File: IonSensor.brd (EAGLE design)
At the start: 50.8 x 22.9 mm, 43 parts, among them IC1 QUAD_OPAMPD, IC2 QUAD_OPAMPD, IC3 QUAD_OPAMPD

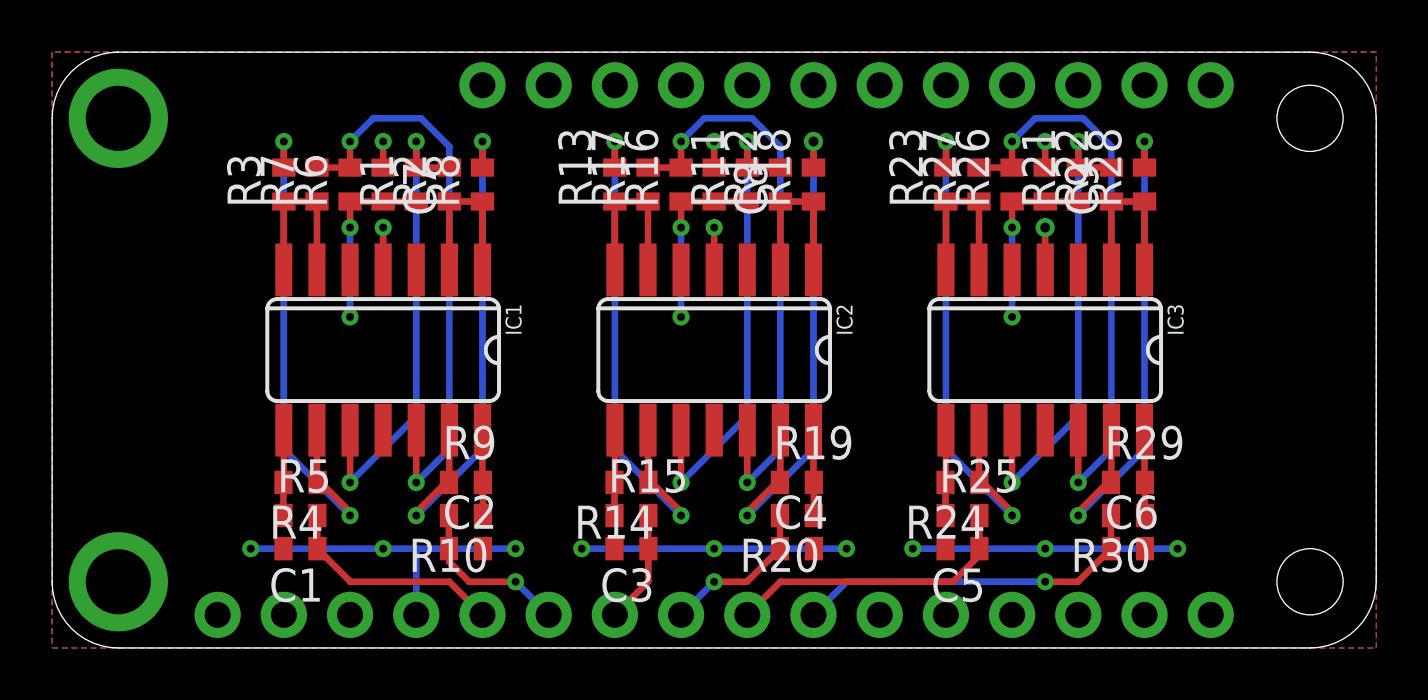
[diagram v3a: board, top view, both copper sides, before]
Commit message: Revert "Rev. D"
This reverts commit b0cd00c38bcd6b0f7db002c888a5e278bdb202ce.
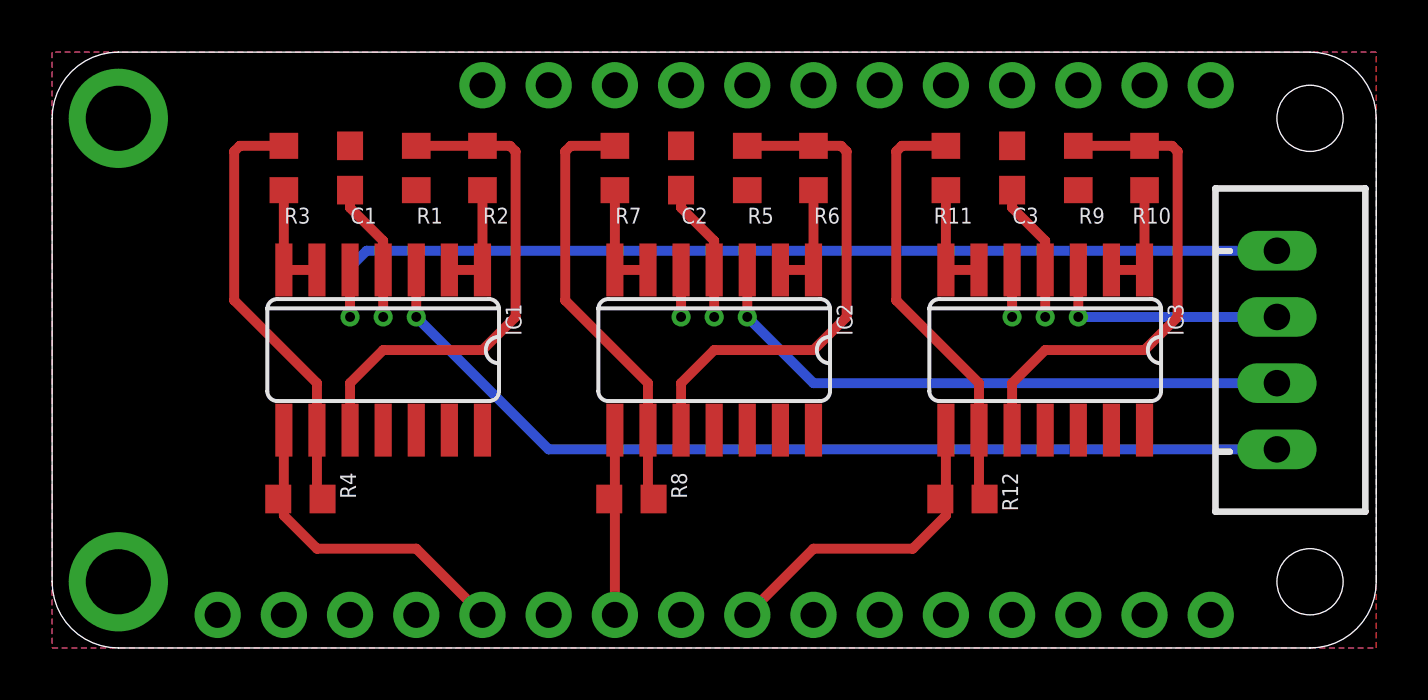
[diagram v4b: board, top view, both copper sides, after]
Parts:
- removed C4, C5, C6, C7, C8, C9: 0.1uF, adafruit:C0402
- removed R13, R17, R18, R22, R23, R27, R28: 10k, adafruit:R0402
- removed R14, R16, R19, R21, R24, R26, R29: 100k, adafruit:R0402
- removed R15, R20, R25, R30: 1M, adafruit:R0402
- added X1: JST-XH-04-PIN-LONG-PAD, Rembrandt Electronics - JST XH Connectors v1-0:JST-XH-04-PACKAGE-LONG-PAD
- C1, C2, C3: device adafruit:C0402 -> adafruit:C0603
- R1, R2, R3, R4, R7, R9: device adafruit:R0402 -> adafruit:R0603
- R10: value 1M -> 10k; device adafruit:R0402 -> adafruit:R0603
- R11, R6: value 100k -> 10k; device adafruit:R0402 -> adafruit:R0603
- R12, R8: value 10k -> 100k; device adafruit:R0402 -> adafruit:R0603
- R5: value 1M -> 100k; device adafruit:R0402 -> adafruit:R0603
- moved R10 29.3 mm to (41.9, 18.4), turned to 90 degrees
- moved R9 26.4 mm to (39.4, 18.4), turned to 90 degrees
- moved R5 21.7 mm to (26.7, 18.4), turned to 90 degrees
- moved C3 20.7 mm to (36.8, 18.4), turned to 90 degrees
- moved R6 17.8 mm to (29.2, 18.4)
- moved C2 16.8 mm to (24.1, 18.4), turned to 90 degrees
- moved C1 14.7 mm to (11.4, 18.4), turned to 90 degrees
- moved R12 13.9 mm to (34.9, 5.71), turned to 180 degrees
- moved R8 13.4 mm to (22.2, 5.71), turned to 180 degrees
- moved R7 11.4 mm to (21.6, 18.4)
- moved R11 7.65 mm to (34.3, 18.4)
- moved R2 1.42 mm to (16.5, 18.4)
- moved R4 0.63 mm to (9.53, 5.71)
- moved R1 0.63 mm to (14.0, 18.4)
- moved R3 0.63 mm to (8.89, 18.4)
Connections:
- removed net A1: C2.1, MS1.6, R10.2
- removed net A3: C4.1, MS1.8, R20.2
- removed net A5: C6.1, MS1.10, R30.2
- removed net C1+: IC1.1, IC1.2, R2.1, R8.1
- removed net C1-: IC1.6, IC1.7, R3.1, R7.1
- removed net C2+: IC2.1, IC2.2, R12.1, R18.1
- removed net C2-: IC2.6, IC2.7, R13.1, R17.1
- removed net C3+: IC3.1, IC3.2, R22.1, R28.1
- removed net C3-: IC3.6, IC3.7, R23.1, R27.1
- removed net N$10: IC1.14, R10.1, R9.2
- removed net N$15: IC3.13, R28.2, R29.1
- removed net N$16: IC2.14, R19.2, R20.1
- removed net N$17: IC3.8, R24.2, R25.1
- removed net N$18: IC3.14, R29.2, R30.1
- removed net N$4 (its old number): IC1.12, R6.2, R7.2
- removed net N$5: IC1.8, R4.2, R5.1
- new net N$1: IC1.1, IC1.2, R2.1
- net +3V3: now also C1.1, C2.1, C3.1; no longer C7.1, C8.1, C9.1
- net A0: now also IC1.8, R4.2; no longer C1.1, R5.2
- net A2: now also IC2.8, R8.2; no longer C3.1, R15.2
- net A4: now also IC3.8, R12.2; no longer C5.1, R25.2
- net CH0: now also X1.4
- net CH1: now also X1.3
- net CH2: now also X1.2
- net GND: now also R5.1, R9.1; no longer C4.2, C5.2, C6.2, C7.2, C8.2, C9.2, R11.1, R16.1, R21.1, R26.1, R6.1
- net N$11: now also IC3.1, IC3.2, R10.1; no longer IC2.12, R16.2, R17.2
- net N$12: now also IC3.6, IC3.7, R11.1; no longer IC3.12, R26.2, R27.2
- net N$13: now also IC3.10, R10.2, R9.2; no longer IC2.13, R18.2, R19.1
- net N$14: now also IC3.9, R11.2, R12.1; no longer IC2.8, R14.2, R15.1
- net N$3: now also IC1.6, IC1.7, R3.1; no longer IC3.10, R21.2, R22.2
- net N$6: now also IC2.1, IC2.2, R6.1; no longer IC1.13, R8.2, R9.1
- net N$7: now also IC2.6, IC2.7, R7.1; no longer IC3.9, R23.2, R24.1
- net N$8: now also R5.2, R6.2; no longer R11.2, R12.2
- net N$9: now also R7.2, R8.1; no longer R13.2, R14.1
- net REF: now also X1.1
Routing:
- net GND: track 53.9 -> 0.00 mm, vias 15 -> 0
- net REF: track 0.00 -> 48.2 mm, vias 0 -> 3
- net CH0: track 0.00 -> 36.9 mm, vias 0 -> 1
- net CH1: track 0.00 -> 23.2 mm, vias 0 -> 1
- net N$4 (its old number): track 22.3 -> 0.00 mm, vias 2 -> 0
- net N$15: track 20.3 -> 0.00 mm, vias 2 -> 0
- net N$11: track 22.3 -> 4.33 mm, vias 2 -> 0
- net N$12: track 22.3 -> 4.33 mm, vias 2 -> 0
- net N$7: track 20.3 -> 4.33 mm, vias 2 -> 0
- net N$6: track 20.3 -> 4.33 mm, vias 2 -> 0
- net N$3: track 18.4 -> 4.33 mm, vias 2 -> 0
- net A5: track 13.7 -> 0.00 mm, vias 1 -> 0
- net N$14: track 3.28 -> 16.7 mm
- net CH2: track 0.00 -> 9.42 mm, vias 0 -> 1
- net +3V3: track 7.88 -> 16.2 mm, vias 6 -> 3
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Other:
- board text removed: "Rev. D"

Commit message: Revert "Fixed wiring"
This reverts commit 887158206b74e515af25e9af216689274ec85624.
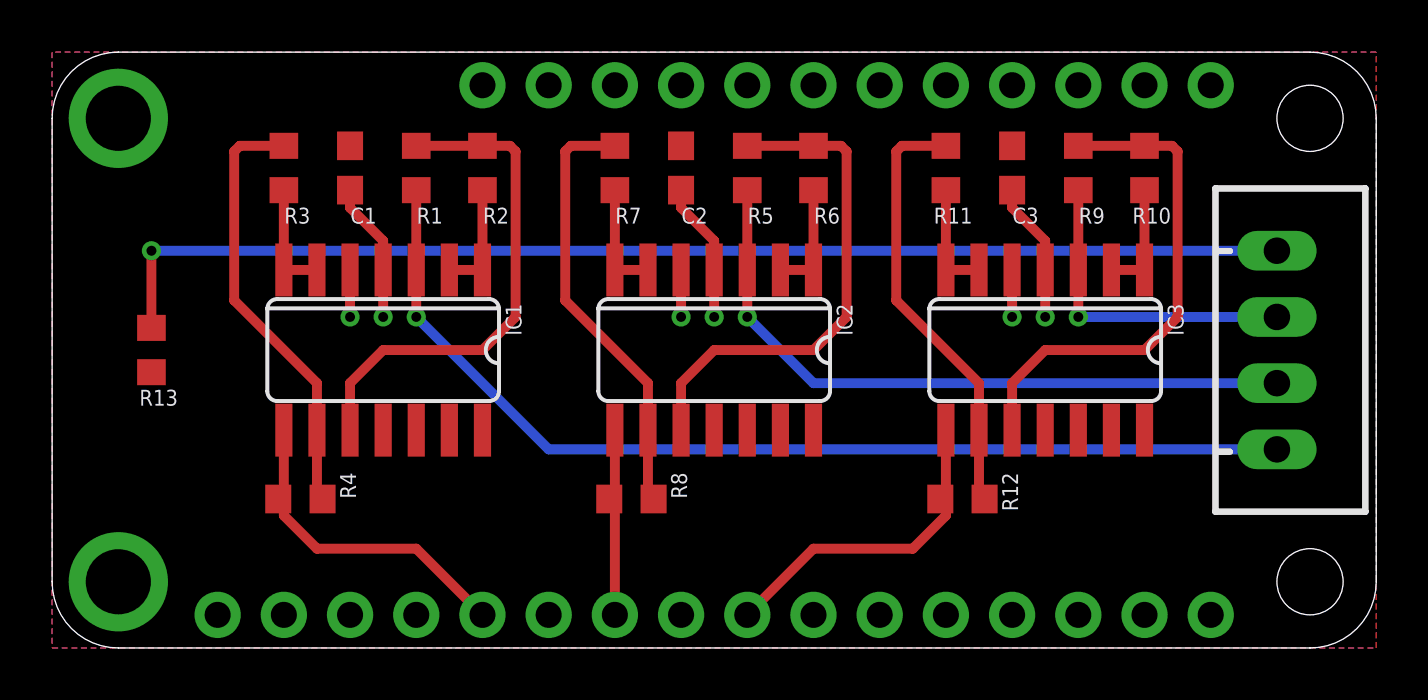
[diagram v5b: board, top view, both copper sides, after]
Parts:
- added R13: 10k, rcl:R0603
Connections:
- net CH0: now also R1.1
- net CH1: now also R5.1
- net CH2: now also R9.1
- net GND: now also R13.2; no longer R1.1, R5.1, R9.1
- net REF: now also R13.1
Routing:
- net REF: track 48.2 -> 59.2 mm, vias 3 -> 4
- net CH2: track 9.42 -> 12.5 mm
- net CH1: track 23.2 -> 26.2 mm
- net CH0: track 36.9 -> 40.0 mm
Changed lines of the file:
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@@
 </element>
 <element name="X1" library="Rembrandt Electronics - JST XH Connectors v1-0" package="JST-XH-04-PACKAGE-LONG-PAD" value="JST-XH-04-PIN-LONG-PAD" x="46.99" y="11.43" smashed="yes" rot="R270"/>
+<element name="R13" library="rcl" library_urn="urn:adsk.eagle:library:334" package="R0603" package3d_urn="urn:adsk.eagle:package:23555/3" value="10k" x="3.81" y="11.43" smashed="yes" rot="R270">
+<attribute name="NAME" x="4.826" y="9.906" size="0.6096" layer="25" rot="R180"/>
+<attribute name="POPULARITY" value="77" x="3.81" y="11.43" size="1.778" layer="27" ratio="15" rot="R270" display="off"/>
+<attribute name="SPICEPREFIX" value="R" x="3.81" y="11.43" size="1.778" layer="27" ratio="15" rot="R270" display="off"/>
+<attribute name="VALUE" x="2.794" y="12.954" size="0.6096" layer="27"/>
+</element>
 </elements>
 <signals>
@@
 <contactref element="C2" pad="2"/>
 <contactref element="C1" pad="2"/>
-<contactref element="R1" pad="1"/>
-<contactref element="R5" pad="1"/>
-<contactref element="R9" pad="1"/>
+<contactref element="R13" pad="2"/>
 </signal>
 <signal name="+3V3">
@@
 <signal name="CH0">
 <contactref element="IC1" pad="3"/>
+<contactref element="R1" pad="1"/>
+<wire x1="13.97" y1="14.5034" x2="13.97" y2="17.565" width="0.381" layer="1"/>
 <wire x1="13.97" y1="14.5034" x2="13.97" y2="12.7" width="0.381" layer="1"/>
 <via x="13.97" y="12.7" extent="1-16" drill="0.381"/>
@@
 <signal name="CH1">
 <contactref element="IC2" pad="3"/>
+<contactref element="R5" pad="1"/>
+<wire x1="26.67" y1="17.565" x2="26.67" y2="14.5034" width="0.381" layer="1"/>
 <wire x1="26.67" y1="14.5034" x2="26.67" y2="12.7" width="0.381" layer="1"/>
 <via x="26.67" y="12.7" extent="1-16" drill="0.381"/>
@@
 <signal name="CH2">
 <contactref element="IC3" pad="3"/>
+<contactref element="R9" pad="1"/>
+<wire x1="39.37" y1="14.5034" x2="39.37" y2="17.565" width="0.381" layer="1"/>
 <wire x1="39.37" y1="14.5034" x2="39.37" y2="12.7" width="0.381" layer="1"/>
 <via x="39.37" y="12.7" extent="1-16" drill="0.381"/>
@@
 <contactref element="IC1" pad="5"/>
 <contactref element="IC2" pad="5"/>
+<contactref element="R13" pad="1"/>
 <wire x1="11.43" y1="14.5034" x2="11.43" y2="12.7" width="0.381" layer="1"/>
 <via x="11.43" y="12.7" extent="1-16" drill="0.381"/>
@@
 <wire x1="36.83" y1="14.5034" x2="36.83" y2="12.7" width="0.381" layer="1"/>
 <via x="36.83" y="12.7" extent="1-16" drill="0.381"/>
-<wire x1="11.43" y1="12.7" x2="11.43" y2="14.605" width="0.381" layer="16"/>
-<wire x1="12.065" y1="15.24" x2="11.43" y2="14.605" width="0.381" layer="16"/>
-<wire x1="12.065" y1="15.24" x2="24.13" y2="15.24" width="0.381" layer="16"/>
+<wire x1="3.81" y1="12.28" x2="3.81" y2="15.24" width="0.381" layer="1"/>
+<via x="3.81" y="15.24" extent="1-16" drill="0.381"/>
+<wire x1="3.81" y1="15.24" x2="11.43" y2="15.24" width="0.381" layer="16"/>
+<wire x1="11.43" y1="15.24" x2="24.13" y2="15.24" width="0.381" layer="16"/>
 <wire x1="24.13" y1="15.24" x2="36.83" y2="15.24" width="0.381" layer="16"/>
+<wire x1="11.43" y1="12.7" x2="11.43" y2="15.24" width="0.381" layer="16"/>
 <wire x1="24.13" y1="12.7" x2="24.13" y2="15.24" width="0.381" layer="16"/>
 <wire x1="36.83" y1="12.7" x2="36.83" y2="15.24" width="0.381" layer="16"/>

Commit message: Fixed wiring
Made sure it's a differential amplifier!
Removed R13.
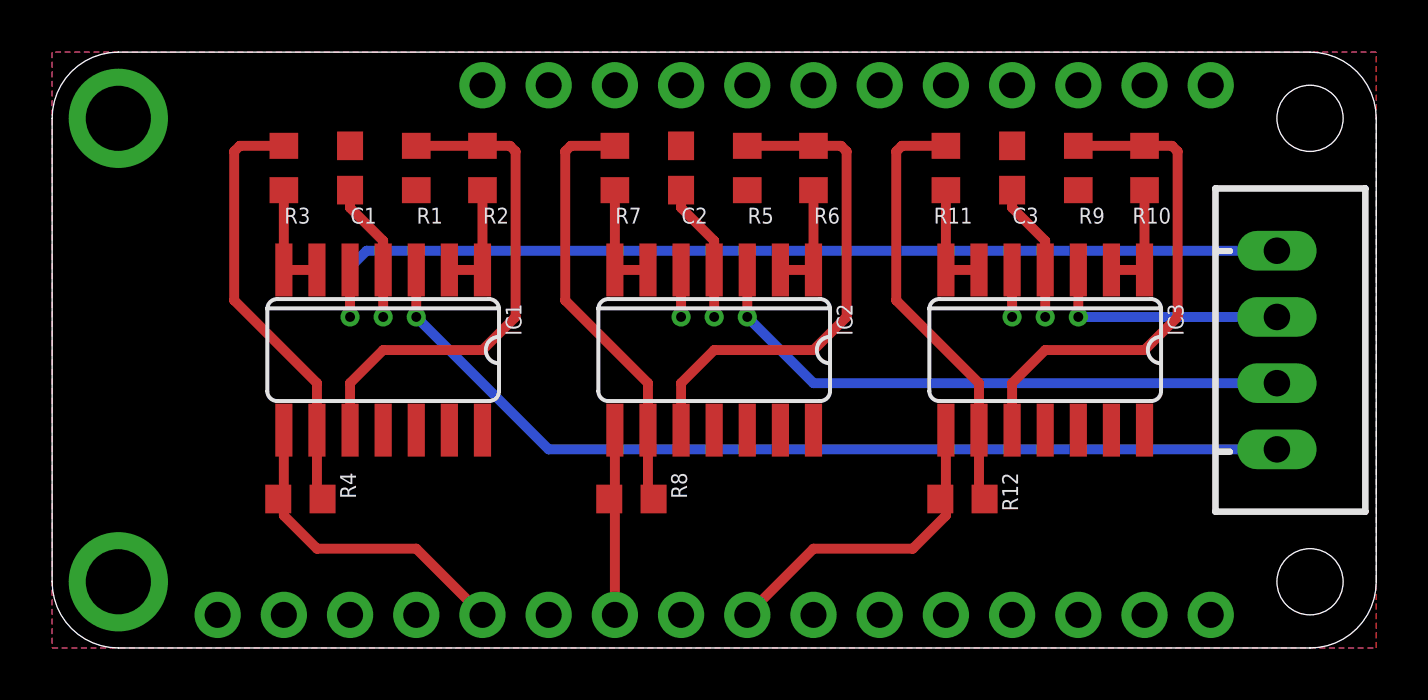
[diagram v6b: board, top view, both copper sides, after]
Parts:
- removed R13: 10k, rcl:R0603
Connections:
- net CH0: no longer R1.1
- net CH1: no longer R5.1
- net CH2: no longer R9.1
- net GND: now also R1.1, R5.1, R9.1; no longer R13.2
- net REF: no longer R13.1
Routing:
- net REF: track 59.2 -> 48.2 mm, vias 4 -> 3
- net CH2: track 12.5 -> 9.42 mm
- net CH1: track 26.2 -> 23.2 mm
- net CH0: track 40.0 -> 36.9 mm
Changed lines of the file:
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@@
 </element>
 <element name="X1" library="Rembrandt Electronics - JST XH Connectors v1-0" package="JST-XH-04-PACKAGE-LONG-PAD" value="JST-XH-04-PIN-LONG-PAD" x="46.99" y="11.43" smashed="yes" rot="R270"/>
-<element name="R13" library="rcl" library_urn="urn:adsk.eagle:library:334" package="R0603" package3d_urn="urn:adsk.eagle:package:23555/3" value="10k" x="3.81" y="11.43" smashed="yes" rot="R270">
-<attribute name="NAME" x="4.826" y="9.906" size="0.6096" layer="25" rot="R180"/>
-<attribute name="POPULARITY" value="77" x="3.81" y="11.43" size="1.778" layer="27" ratio="15" rot="R270" display="off"/>
-<attribute name="SPICEPREFIX" value="R" x="3.81" y="11.43" size="1.778" layer="27" ratio="15" rot="R270" display="off"/>
-<attribute name="VALUE" x="2.794" y="12.954" size="0.6096" layer="27"/>
-</element>
 </elements>
 <signals>
@@
 <contactref element="C2" pad="2"/>
 <contactref element="C1" pad="2"/>
-<contactref element="R13" pad="2"/>
+<contactref element="R1" pad="1"/>
+<contactref element="R5" pad="1"/>
+<contactref element="R9" pad="1"/>
 </signal>
 <signal name="+3V3">
@@
 <signal name="CH0">
 <contactref element="IC1" pad="3"/>
-<contactref element="R1" pad="1"/>
-<wire x1="13.97" y1="14.5034" x2="13.97" y2="17.565" width="0.381" layer="1"/>
 <wire x1="13.97" y1="14.5034" x2="13.97" y2="12.7" width="0.381" layer="1"/>
 <via x="13.97" y="12.7" extent="1-16" drill="0.381"/>
@@
 <signal name="CH1">
 <contactref element="IC2" pad="3"/>
-<contactref element="R5" pad="1"/>
-<wire x1="26.67" y1="17.565" x2="26.67" y2="14.5034" width="0.381" layer="1"/>
 <wire x1="26.67" y1="14.5034" x2="26.67" y2="12.7" width="0.381" layer="1"/>
 <via x="26.67" y="12.7" extent="1-16" drill="0.381"/>
@@
 <signal name="CH2">
 <contactref element="IC3" pad="3"/>
-<contactref element="R9" pad="1"/>
-<wire x1="39.37" y1="14.5034" x2="39.37" y2="17.565" width="0.381" layer="1"/>
 <wire x1="39.37" y1="14.5034" x2="39.37" y2="12.7" width="0.381" layer="1"/>
 <via x="39.37" y="12.7" extent="1-16" drill="0.381"/>
@@
 <contactref element="IC1" pad="5"/>
 <contactref element="IC2" pad="5"/>
-<contactref element="R13" pad="1"/>
 <wire x1="11.43" y1="14.5034" x2="11.43" y2="12.7" width="0.381" layer="1"/>
 <via x="11.43" y="12.7" extent="1-16" drill="0.381"/>
@@
 <wire x1="36.83" y1="14.5034" x2="36.83" y2="12.7" width="0.381" layer="1"/>
 <via x="36.83" y="12.7" extent="1-16" drill="0.381"/>
-<wire x1="3.81" y1="12.28" x2="3.81" y2="15.24" width="0.381" layer="1"/>
-<via x="3.81" y="15.24" extent="1-16" drill="0.381"/>
-<wire x1="3.81" y1="15.24" x2="11.43" y2="15.24" width="0.381" layer="16"/>
-<wire x1="11.43" y1="15.24" x2="24.13" y2="15.24" width="0.381" layer="16"/>
+<wire x1="11.43" y1="12.7" x2="11.43" y2="14.605" width="0.381" layer="16"/>
+<wire x1="12.065" y1="15.24" x2="11.43" y2="14.605" width="0.381" layer="16"/>
+<wire x1="12.065" y1="15.24" x2="24.13" y2="15.24" width="0.381" layer="16"/>
 <wire x1="24.13" y1="15.24" x2="36.83" y2="15.24" width="0.381" layer="16"/>
-<wire x1="11.43" y1="12.7" x2="11.43" y2="15.24" width="0.381" layer="16"/>
 <wire x1="24.13" y1="12.7" x2="24.13" y2="15.24" width="0.381" layer="16"/>
 <wire x1="36.83" y1="12.7" x2="36.83" y2="15.24" width="0.381" layer="16"/>
